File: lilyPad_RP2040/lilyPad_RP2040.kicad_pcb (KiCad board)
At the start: 2 copper layers, 50 x 50 mm, 50 parts, among them J1 Conn_01x02, J10 Conn_01x01, J11 Conn_01x01, J12 Conn_01x01, J13 Conn_01x01, J14 Conn_01x01, J15 Conn_01x01, J16 Conn_01x01, J17 Conn_01x01, J18 Conn_01x01, J19 Conn_01x01, J2 USB_C_Receptacle_USB2.0_14P, J20 Conn_01x01, J21 Conn_01x01, J3 Conn_01x03, J4 Conn_01x01, J5 Conn_01x01, J6 Conn_01x01, J7 Conn_01x01, J8 Conn_01x01, J9 Conn_01x01, U1 RP2040, U2 W25Q128JVS, U3 AMS1117-3.3, Y1 C9002

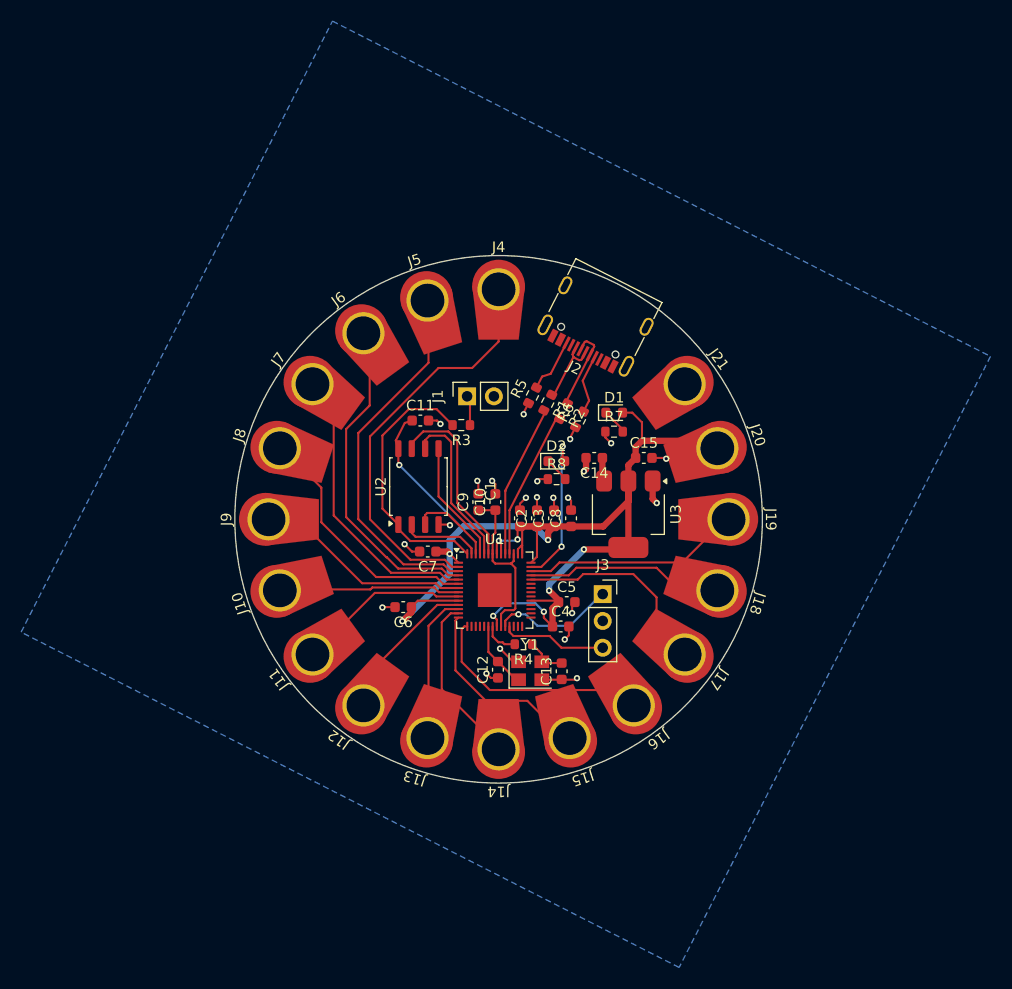
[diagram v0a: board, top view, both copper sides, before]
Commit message: finish_hw
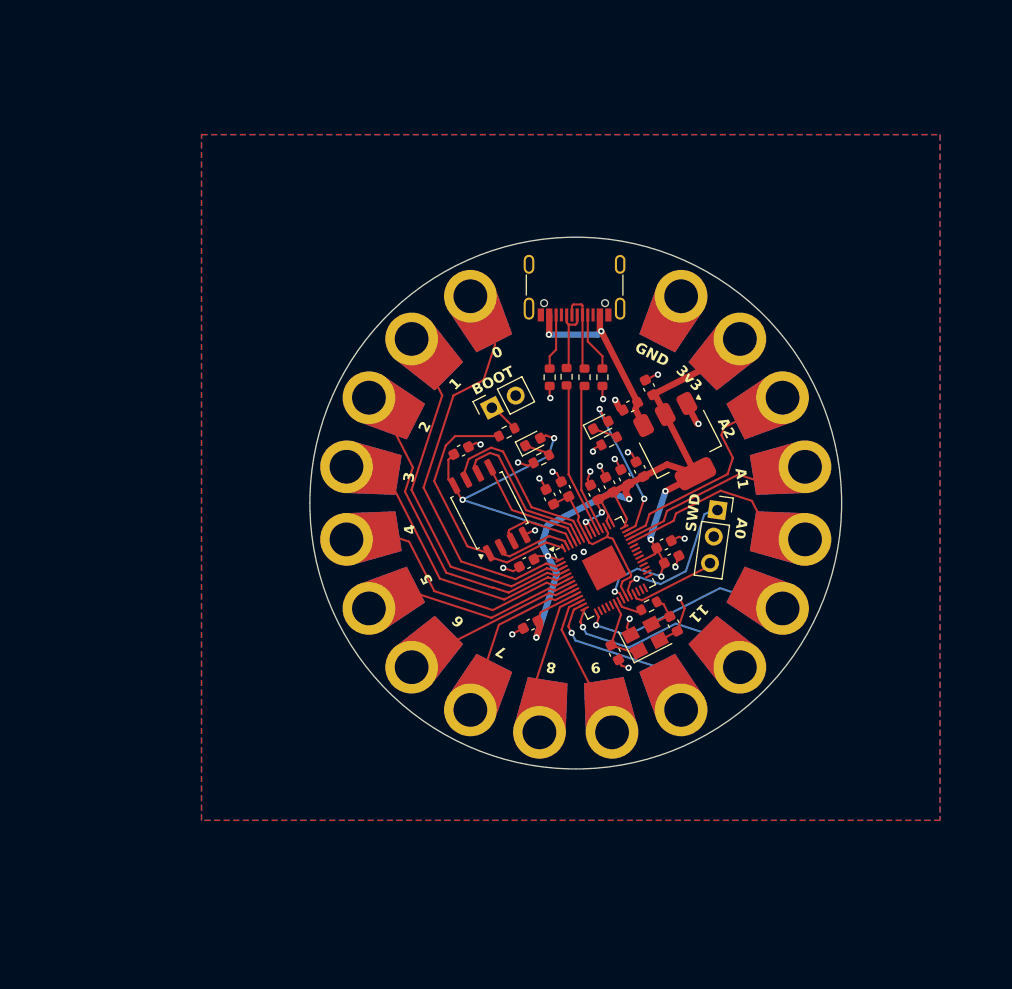
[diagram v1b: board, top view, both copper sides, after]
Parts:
- moved J14 17.5 mm to (149.3, 105.3), turned to -153 degrees
- moved J13 17.3 mm to (142.9, 107.4), turned to -171 degrees
- moved J15 17.3 mm to (154.7, 101.4), turned to -135 degrees
- moved J12 16.7 mm to (136.2, 107.4), turned to 171 degrees
- moved J16 16.6 mm to (158.7, 95.9), turned to -117 degrees
- moved J11 15.8 mm to (129.8, 105.3), turned to 153 degrees
- moved J17 15.5 mm to (160.8, 89.5), turned to -99 degrees
- moved J10 14.4 mm to (124.3, 101.4), turned to 135 degrees
- moved J18 14.1 mm to (160.8, 82.8), turned to -81 degrees
- moved J3 13.5 mm to (153.0, 86.8), turned to -8 degrees
- moved J9 12.7 mm to (120.4, 95.9), turned to 117 degrees
- moved R4 12.4 mm to (146.5, 95.9), turned to -153 degrees
- moved J19 12.3 mm to (158.7, 76.4), turned to -63 degrees
- moved C4 12.3 mm to (148.6, 91.5), turned to 27 degrees
- moved C6 12.2 mm to (135.3, 97.7), turned to -153 degrees
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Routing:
- net VBUS: track 2.25 -> 18.5 mm, vias 0 -> 2
- net /GPIO28_ADC2: track 20.5 -> 25.7 mm
- net +3V3: track 116.8 -> 120.2 mm, vias 10 -> 11
- net /SWCLK: track 11.7 -> 14.2 mm
- net /SWD: track 9.99 -> 8.50 mm
- net GND: track 32.3 -> 33.8 mm, vias 22 -> 24
- net /GPIO11: track 18.4 -> 19.7 mm, vias 0 -> 1
- net /GPIO4: track 23.8 -> 25.0 mm
- net /GPIO10: track 15.9 -> 17.0 mm, vias 0 -> 1
- net /GPIO12: track 21.5 -> 20.5 mm, vias 0 -> 1
- net /XOUT: track 3.36 -> 2.57 mm
- net /XIN: track 6.38 -> 7.06 mm
- net /~{CS}: track 25.3 -> 26.0 mm
- added copper zone on F.Cu, net GND
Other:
- board size 50 x 50 mm -> 50.4 x 50.4 mm
- board text added: "0"
- board text added: "1"
- board text added: "11"
- board text added: "2"
- board text added: "3"
- board text added: "3v3"
- board text added: "4"
- board text added: "5"
- board text added: "6"
- board text added: "7"
- board text added: "8"
- board text added: "9"
- board text added: "A0"
- board text added: "A1"
- board text added: "A2"
- board text added: "BOOT"
- board text added: "GND"
- board text added: "SWD"
- board text added: "lilyPad rp2040"
